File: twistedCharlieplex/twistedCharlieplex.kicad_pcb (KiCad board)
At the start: 6 copper layers, 38.9 x 38.9 mm, 145 parts, among them U2 STM32L412CBUxP

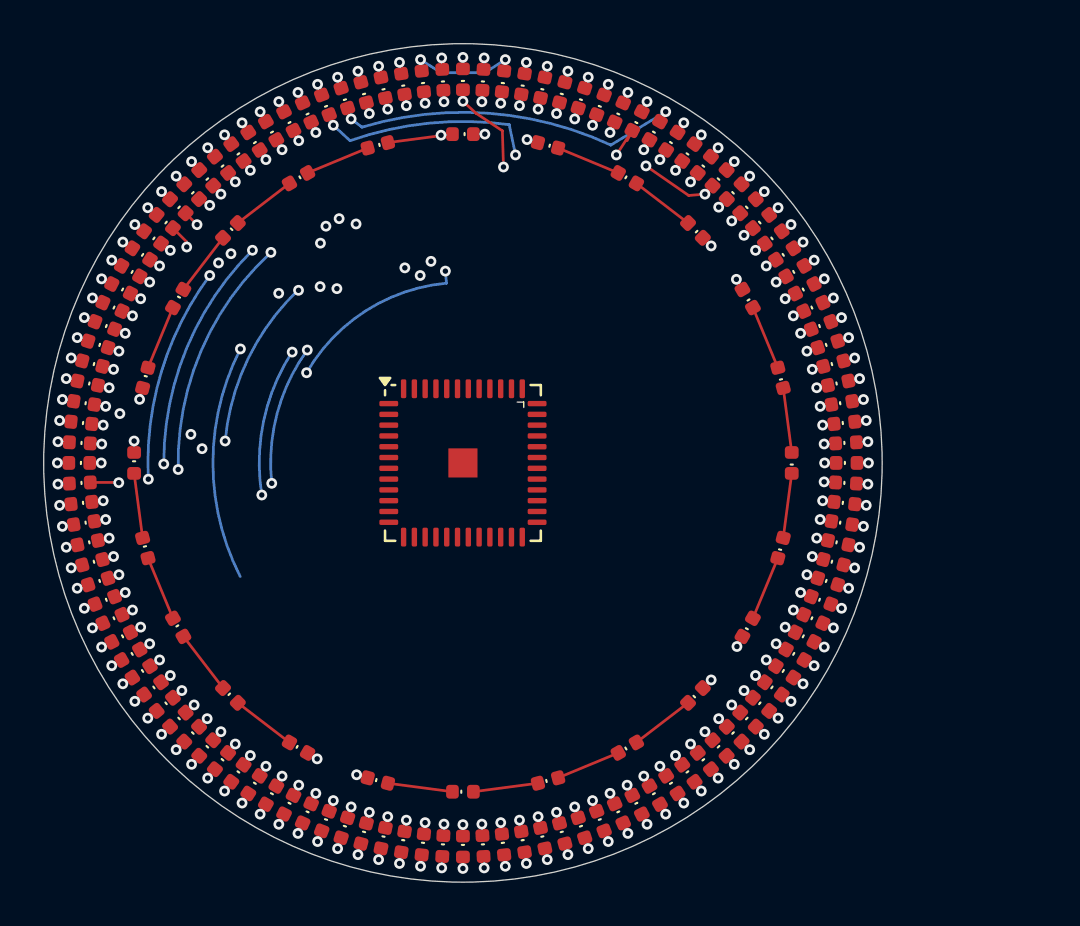
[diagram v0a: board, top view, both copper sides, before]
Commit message: spirograph layout. let the nightmares begin
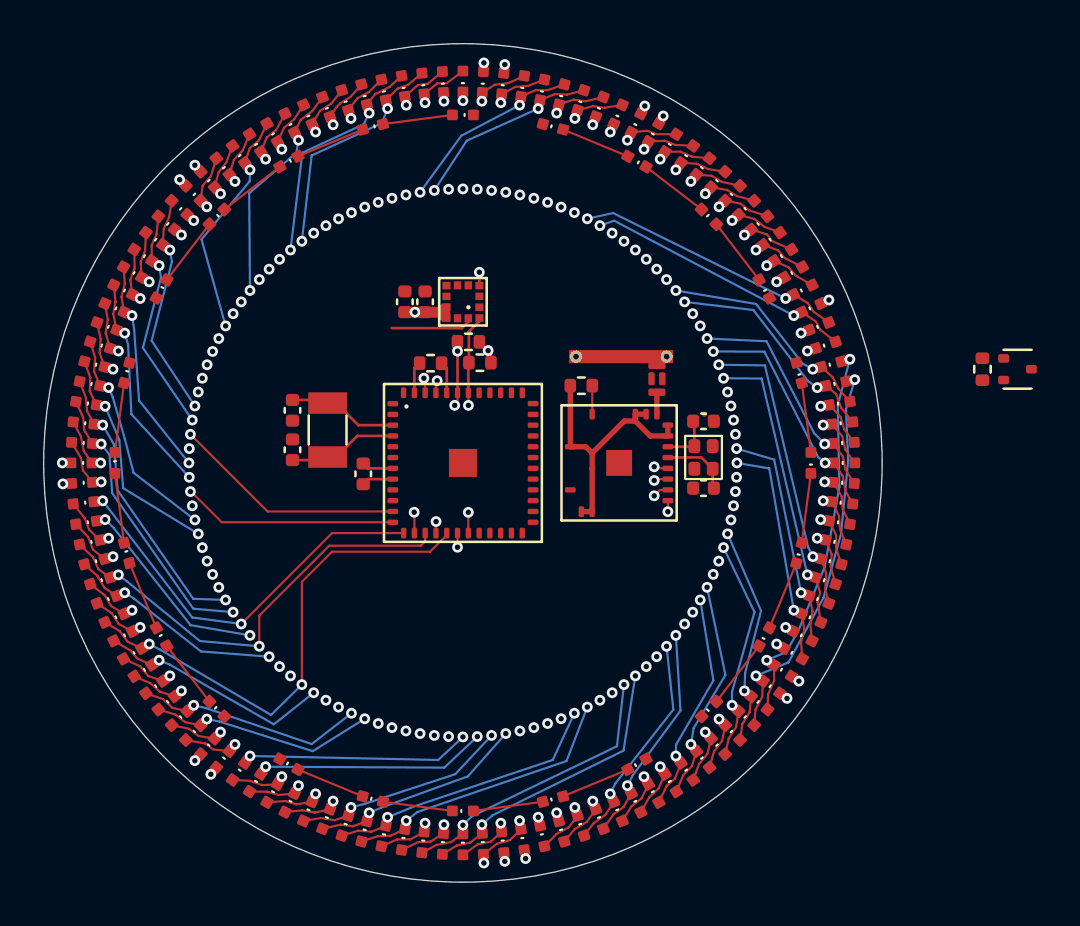
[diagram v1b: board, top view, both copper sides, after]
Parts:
- added AE1: Antenna_Shield, Antenna_SMD:C209892, F.Cu at (8.99, -3.30)
- added C1: 100n, Capacitor_SMD:C_0402_1005Metric, F.Cu at (-1.75, -7.47)
- added C2: 10u, Capacitor_SMD:C_0402_1005Metric, F.Cu at (-2.69, -7.47)
- added C3: 100n, Capacitor_SMD:C_0402_1005Metric, F.Cu at (-4.62, 0.51)
- added C4: 4p3, Capacitor_SMD:C_0402_1005Metric, F.Cu at (-7.90, -2.44)
- added C5: 4p3, Capacitor_SMD:C_0402_1005Metric, F.Cu at (-7.90, -0.61)
- added C6: 12p, Capacitor_SMD:C_0402_1005Metric, F.Cu at (11.2, 1.17)
- added C7: 12p, Capacitor_SMD:C_0402_1005Metric, F.Cu at (11.2, -1.93)
- added Q1: Q_PMOS_GSD, Package_TO_SOT_SMD:SOT-523, F.Cu at (25.7, -4.34)
- added R1: 10k, Resistor_SMD:R_0402_1005Metric, F.Cu at (-1.50, -4.62)
- added R2: 10k, Resistor_SMD:R_0402_1005Metric, F.Cu at (0.79, -4.65)
- added R3: 10k, Resistor_SMD:R_0402_1005Metric, F.Cu at (0.25, -5.61)
- added R4: 100k, Resistor_SMD:R_0402_1005Metric, F.Cu at (5.49, -3.58)
- added R5: 1M, Resistor_SMD:R_0402_1005Metric, F.Cu at (24.1, -4.34)
- added U1: STM32L412CBUx, Package_DFN_QFN:QFN-48-1EP_7x7mm_P0.5mm_EP5.6x5.6mm, F.Cu at (0.00, 0.00)
- added U3: ESP32-C3, Package_DFN_QFN:QFN-32-1EP_5x5mm_P0.5mm_EP3.7x3.7mm, F.Cu at (7.24, 0.00)
- added Y1: 32.768k, Crystal:Crystal_SMD_3215-2Pin_3.2x1.5mm, F.Cu at (-6.27, -1.52)
- added Y2: 40M, SMD_Crystal:Crystal_SMD_1612_4P, F.Cu at (11.2, -0.25)
- U2: value STM32L412CBUxP -> LIS2DW12; footprint Package_DFN_QFN:QFN-48-1EP_7x7mm_P0.5mm_EP5.6x5.6mm -> Package_LGA:LGA-12_2x2mm_P0.5mm
- moved U2 7.47 mm to (0.00, -7.47), turned to 180 degrees
- moved D122 4.19 mm to (-4.17, -15.6), turned to -165 degrees
- moved D128 4.19 mm to (-15.6, 4.17), turned to -75 degrees
- moved D134 4.19 mm to (4.17, 15.6), turned to 15 degrees
- moved D140 4.19 mm to (15.6, -4.17), turned to 105 degrees
- moved D121 4.19 mm to (0.00, -16.1), turned to 180 degrees
- moved D127 4.19 mm to (-16.1, 0.00), turned to -90 degrees
- moved D133 4.19 mm to (0.00, 16.1), turned to 0 degrees
- moved D139 4.19 mm to (16.1, 0.00), turned to 90 degrees
- moved D123 4.19 mm to (-8.06, -14.0), turned to -150 degrees
- moved D129 4.19 mm to (-14.0, 8.06), turned to -60 degrees
- moved D135 4.19 mm to (8.06, 14.0), turned to 30 degrees
- moved D141 4.19 mm to (14.0, -8.06), turned to 120 degrees
- moved D125 4.19 mm to (-14.0, -8.06), turned to -120 degrees
- moved D131 4.19 mm to (-8.06, 14.0), turned to -30 degrees
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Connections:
- net /Charlie Displays/IO0 renamed IO0
- net /Charlie Displays/IO1 renamed IO1
- net /Charlie Displays/IO10 renamed IO10
- net /Charlie Displays/IO11 renamed IO11
- net /Charlie Displays/IO12 renamed IO12
- net /Charlie Displays/IO13 renamed IO13
- net /Charlie Displays/IO14 renamed IO14
- net /Charlie Displays/IO15 renamed IO15
- net /Charlie Displays/IO16 renamed IO16
- net /Charlie Displays/IO17 renamed IO17
- net /Charlie Displays/IO18 renamed IO18
- net /Charlie Displays/IO2 renamed IO2
- net /Charlie Displays/IO20 renamed IO20
- net /Charlie Displays/IO21 renamed IO21
- net /Charlie Displays/IO22 renamed IO22
- net /Charlie Displays/IO23 renamed IO23
- net /Charlie Displays/IO24 renamed IO24
- net /Charlie Displays/IO25 renamed IO25
- net /Charlie Displays/IO3 renamed IO3
- net /Charlie Displays/IO4 renamed IO4
- net /Charlie Displays/IO5 renamed IO5
- net /Charlie Displays/IO6 renamed IO6
- net /Charlie Displays/IO7 renamed IO7
- net /Charlie Displays/IO8 renamed IO8
- U2 pad 1: VCC -> SCL
- U2 pad 10: unconnected-(U2-PA0-Pad10) -> +3V0
- U2 pad 12: unconnected-(U2-PA2-Pad12) -> WKUP1
- U2 pad 4: unconnected-(U2-PC15-Pad4) -> SDA
- U2 pad 6: unconnected-(U2-PH1-Pad6) -> GND
- U2 pad 7: unconnected-(U2-NRST-Pad7) -> GND
- U2 pad 9: VCC -> +3V0
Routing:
- net IO14: track 33.0 -> 146.0 mm, vias 15 -> 17
- net IO6: track 37.6 -> 146.9 mm, vias 15 -> 16
- net IO3: track 23.7 -> 130.1 mm, vias 12 -> 13
- net IO15: track 29.6 -> 131.3 mm, vias 14 -> 13
- net IO4: track 33.8 -> 135.5 mm, vias 15 -> 16
- net IO5: track 28.5 -> 129.0 mm, vias 14 -> 13
- net IO10: track 20.7 -> 121.0 mm, vias 13 -> 14
- net IO0: track 38.8 -> 138.2 mm, vias 15 -> 14
- net IO13: track 29.8 -> 119.7 mm, vias 13 -> 12
- net IO16: track 36.6 -> 126.3 mm, vias 15 -> 16
- net IO17: track 36.2 -> 122.9 mm, vias 16 -> 15
- net IO7: track 38.4 -> 124.7 mm, vias 16 -> 14
- net IO1: track 51.5 -> 136.4 mm, vias 16 -> 14
- net IO2: track 48.9 -> 130.0 mm, vias 16 -> 15
- net IO18: track 44.1 -> 123.9 mm, vias 18 -> 15
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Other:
- copper layers 6 -> 4
